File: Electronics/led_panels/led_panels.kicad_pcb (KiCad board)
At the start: 2 copper layers, 160 x 100 mm, 118 parts, among them P1 CONN_2

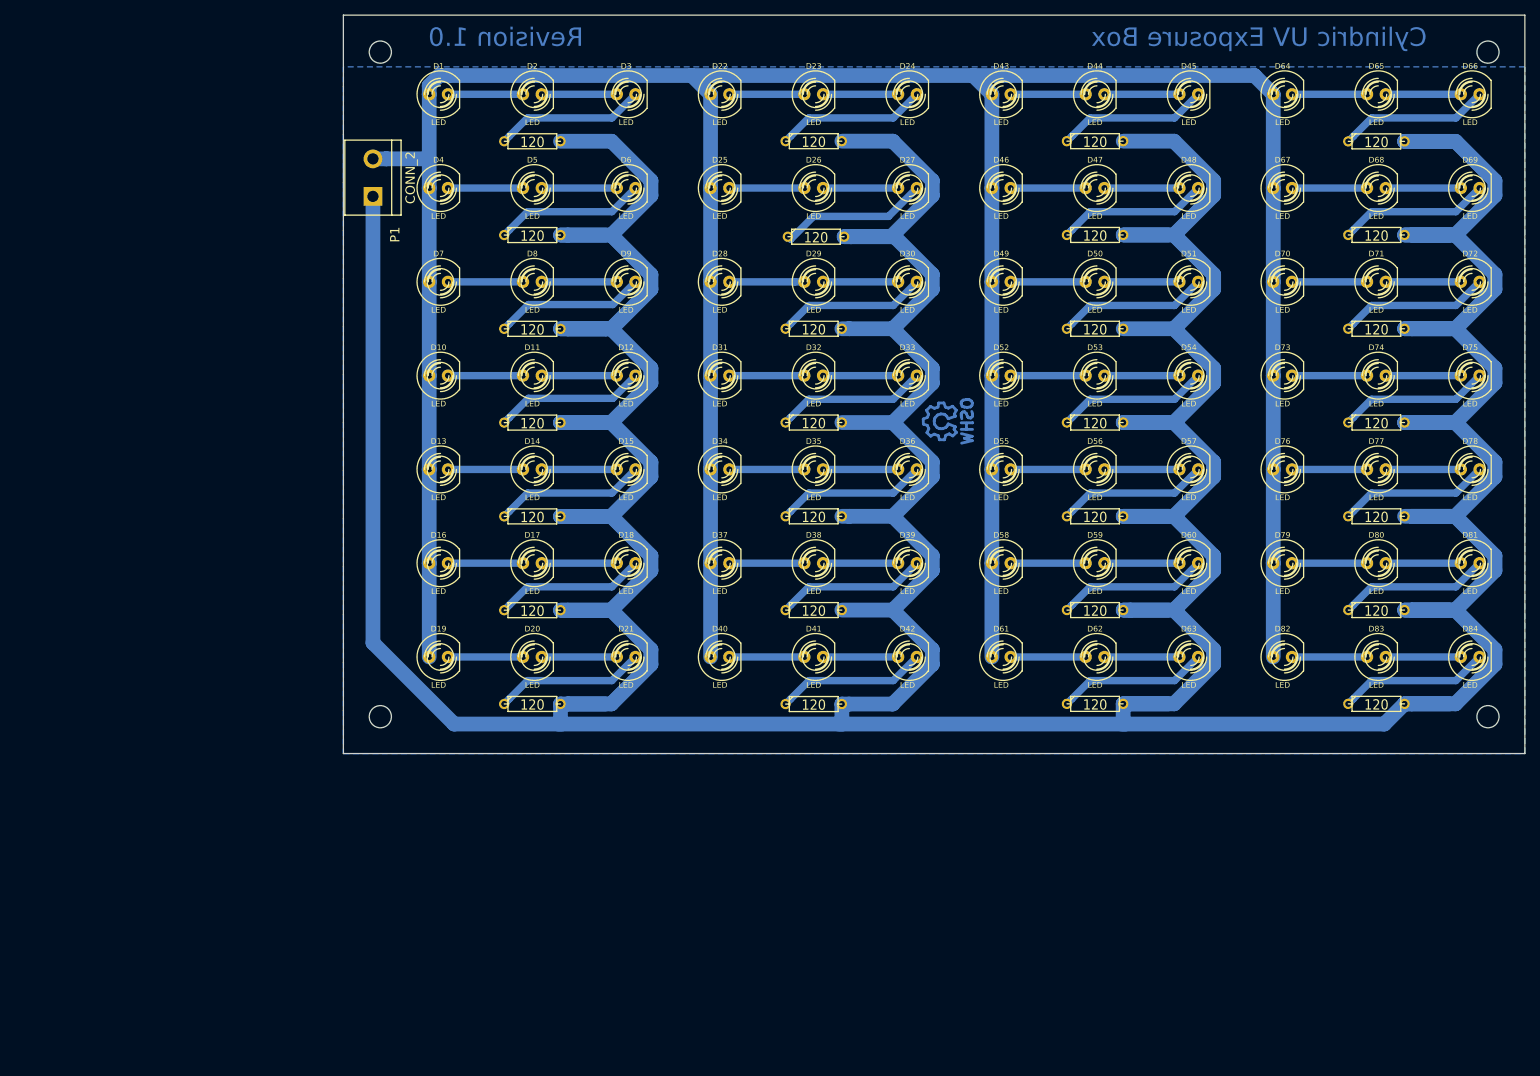
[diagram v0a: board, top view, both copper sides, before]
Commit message: Moved some parts around on the board.
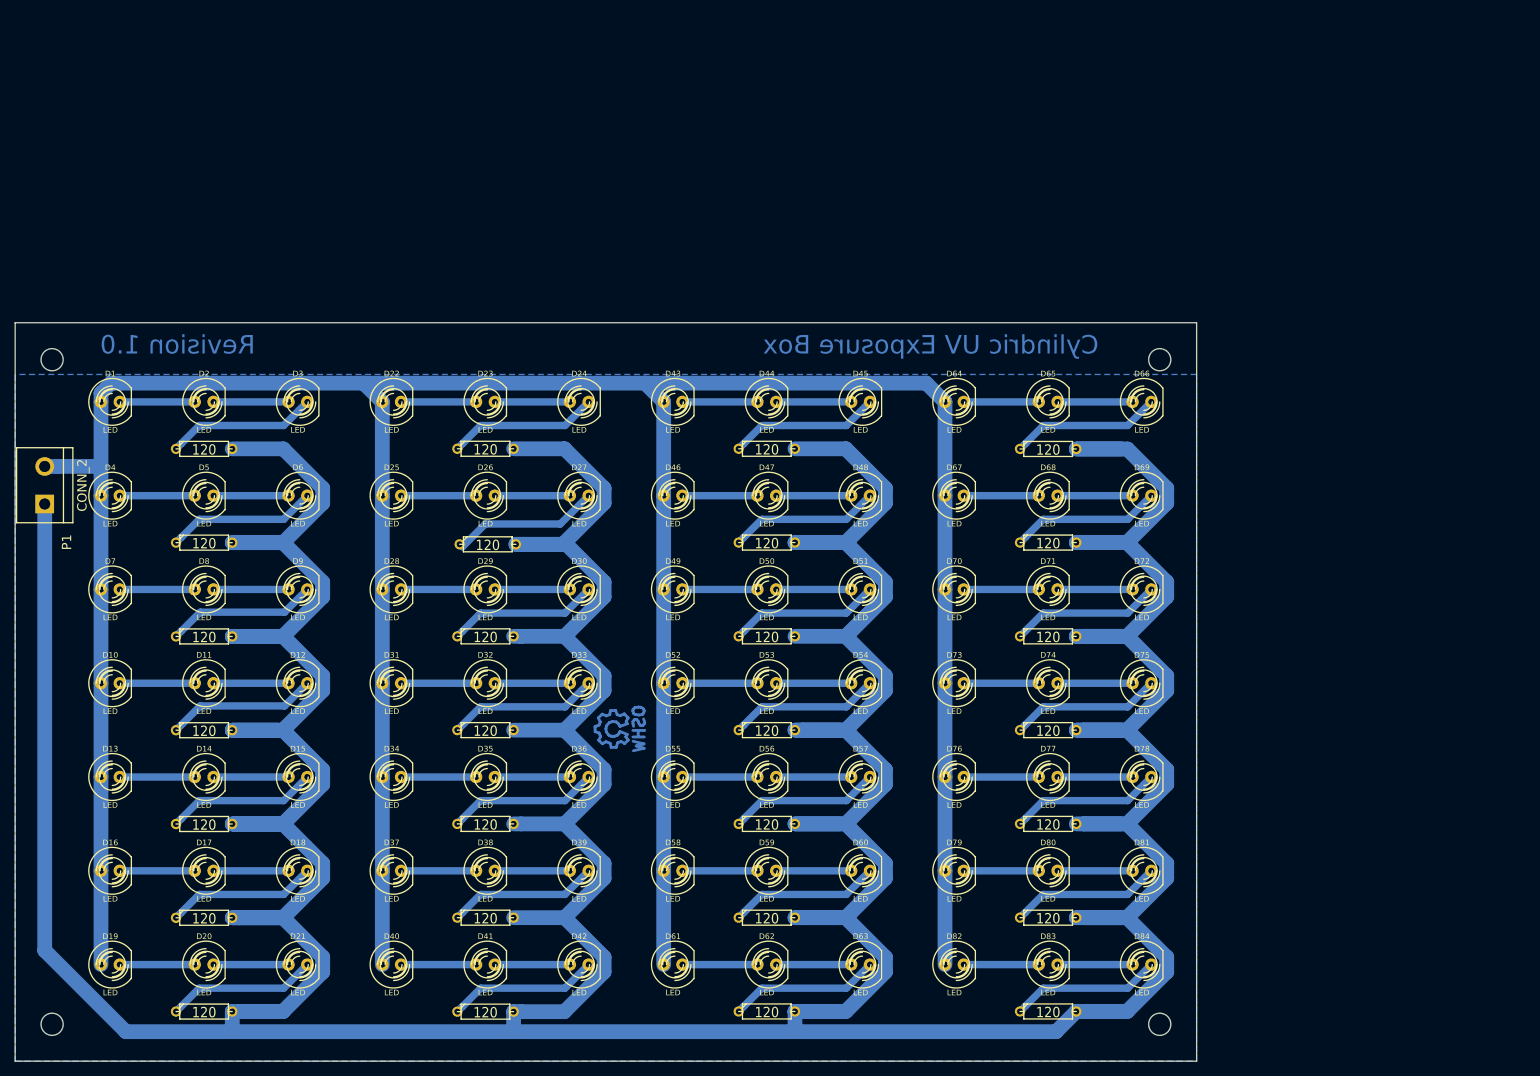
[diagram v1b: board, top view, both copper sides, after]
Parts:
- moved D26 60.9 mm to (85.7, 111.1)
- moved D29 60.9 mm to (85.7, 123.8)
- moved D32 60.9 mm to (85.7, 136.5)
- moved D38 60.9 mm to (85.7, 161.9)
- moved D41 60.9 mm to (85.7, 174.6)
- moved D67 60.9 mm to (149.2, 111.1)
- moved D70 60.9 mm to (149.2, 123.8)
- moved D73 60.9 mm to (149.2, 136.5)
- moved D79 60.9 mm to (149.2, 161.9)
- moved D82 60.9 mm to (149.2, 174.6)
- moved MountingHole_3mm 60.9 mm to (177.0, 182.7)
- moved R10 60.9 mm to (85.7, 130.2)
- moved R11 60.9 mm to (85.7, 142.9)
- moved R13 60.9 mm to (85.7, 168.3)
- moved R14 60.9 mm to (85.7, 181.0)
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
